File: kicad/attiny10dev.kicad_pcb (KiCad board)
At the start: 2 copper layers, 19 parts, among them J1 Conn_02x06_Odd_Even, J2 Conn_01x06, J3 Conn_01x03_Male, K1 m4-12h, K2 m4-12h, Q1 2N7002, Q2 BSS84, Q3 2N7002, Q4 FZT600, Q5 2N7002, U1 ATtiny10-TS, U2 ATtiny10-TS

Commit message: Work on next gen pcb
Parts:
- added C10: 100n, Capacitor_SMD:C_0805_2012Metric_Pad1.15x1.40mm_HandSolder, F.Cu at (239.3, 85.1)
- added C11: 500p, Capacitor_SMD:C_0805_2012Metric_Pad1.15x1.40mm_HandSolder, F.Cu at (259.4, 81.6)
- added C12: 470u, Capacitor_THT:CP_Radial_D8.0mm_P5.00mm, F.Cu at (254.3, 105.8)
- added C4: 1u, Capacitor_SMD:C_0805_2012Metric_Pad1.15x1.40mm_HandSolder, F.Cu at (233.8, 92.5)
- added C5: 100n, Capacitor_SMD:C_0805_2012Metric_Pad1.15x1.40mm_HandSolder, F.Cu at (243.7, 67.6)
- added C6: 100n, Capacitor_SMD:C_0805_2012Metric_Pad1.15x1.40mm_HandSolder, F.Cu at (250.8, 96.8)
- added C7: 100n, Capacitor_SMD:C_0805_2012Metric_Pad1.15x1.40mm_HandSolder, F.Cu at (246.6, 85.2)
- added C8: 100n, Capacitor_SMD:C_0805_2012Metric_Pad1.15x1.40mm_HandSolder, F.Cu at (237.6, 101.1)
- added C9: 470u, Capacitor_THT:CP_Radial_D8.0mm_P5.00mm, F.Cu at (263.6, 105.8)
- added D2: D, Diode_SMD:D_3220_8050Metric_Pad2.65x5.15mm_HandSolder, F.Cu at (259.5, 89.8)
- added F1: 500ma, Fuse:Fuse_1206_3216Metric_Pad1.42x1.75mm_HandSolder, F.Cu at (231.2, 95.9)
- added L1: 33u, Inductor_THT:L_Toroid_Vertical_L13.0mm_W6.5mm_P5.60mm, F.Cu at (272.8, 91.5)
- added R10: 10k, Capacitor_SMD:C_0603_1608Metric_Pad1.05x0.95mm_HandSolder, F.Cu at (254.2, 97.8)
- added R4: 10k, Capacitor_SMD:C_0603_1608Metric_Pad1.05x0.95mm_HandSolder, F.Cu at (217.7, 105.5)
- added R5: 22, Capacitor_SMD:C_0603_1608Metric_Pad1.05x0.95mm_HandSolder, F.Cu at (229.6, 90.7)
- added R6: 22, Capacitor_SMD:C_0603_1608Metric_Pad1.05x0.95mm_HandSolder, F.Cu at (229.6, 89.0)
- added R7: 470m, Resistor_THT:R_Axial_DIN0204_L3.6mm_D1.6mm_P2.54mm_Vertical, F.Cu at (258.3, 97.6)
- added R8: 180, Capacitor_SMD:C_0603_1608Metric_Pad1.05x0.95mm_HandSolder, F.Cu at (263.8, 98.6)
- added R9: 86k, Capacitor_SMD:C_0603_1608Metric_Pad1.05x0.95mm_HandSolder, F.Cu at (256.0, 97.8)
- added SW1: SW_Push, Button_Switch_THT:SW_PUSH_6mm, F.Cu at (220.2, 101.5)
- added U3: ATmega32U4-AU, Package_QFP:TQFP-44_10x10mm_P0.8mm, F.Cu at (243.0, 93.0)
- added U4: MC34063AD, Package_DIP:DIP-8_W10.16mm, F.Cu at (263.3, 84.7)
- added Y1: 16Mhz, Crystal:Crystal_SMD_HC49-SD, F.Cu at (242.9, 104.9)
- C2, C3: value 22u -> 22p; footprint Capacitor_THT:CP_Radial_D12.5mm_P5.00mm -> Capacitor_SMD:C_0805_2012Metric_Pad1.15x1.40mm_HandSolder; moved to F.Cu
- D1, J1, K1, K2, U2: moved to F.Cu
- J2: value Conn_01x06 -> Conn_02x03_Odd_Even; footprint Connector_PinHeader_2.54mm:PinHeader_1x06_P2.54mm_Vertical -> Connector_PinHeader_2.54mm:PinHeader_2x03_P2.54mm_Vertical; moved to F.Cu
- J3: value Conn_01x03_Male -> USB_B; footprint TerminalBlock_RND:TerminalBlock_RND_205-00277_1x03_P5.00mm_Vertical -> Connector_USB:USB_B_OST_USB-B1HSxx_Horizontal; moved to F.Cu
- Q4: value FZT600 -> 2N7002; footprint Package_TO_SOT_THT:TO-92 -> Package_TO_SOT_SMD:SOT-23; moved to F.Cu
- R1, R2, R3: footprint Resistor_SMD:R_0805_2012Metric_Pad1.15x1.40mm_HandSolder -> Capacitor_SMD:C_0603_1608Metric_Pad1.05x0.95mm_HandSolder
- moved K2 216.4 mm to (268.6, 69.3), turned to 0 degrees
- moved J2 194.5 mm to (231.1, 100.2)
- moved C3 193.4 mm to (241.1, 101.1)
- moved Q5 192.8 mm to (232.0, 80.2), turned to 90 degrees
- moved K1 191.9 mm to (256.2, 69.9), turned to 0 degrees
- moved R1 190.4 mm to (229.3, 76.4), turned to 270 degrees
- moved R3 188.3 mm to (232.2, 77.0), turned to 180 degrees
- moved Q1 185.6 mm to (223.8, 80.3), turned to 90 degrees
- moved Q3 185.5 mm to (228.0, 80.3), turned to 0 degrees
- moved Q2 183.8 mm to (226.2, 76.5), turned to 180 degrees
- moved C1 179.5 mm to (259.3, 100.1), turned to 0 degrees
- moved D1 175.2 mm to (231.6, 74.7), turned to 0 degrees
- moved C2 175.2 mm to (244.6, 101.1)
- moved Q4 171.3 mm to (236.1, 78.2), turned to 90 degrees
- moved J3 168.1 mm to (224.8, 92.2), turned to 180 degrees
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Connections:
- C2 pad 1: GND -> Net-(C2-Pad1)
- C2 pad 2: +5V -> GND
- C3 pad 1: GND -> Net-(C3-Pad1)
- C3 pad 2: +12V -> GND
- J2 pad 1: /tpidata -> /prog_miso
- J2 pad 2: /tpiclk -> +5V
- J2 pad 3: /prog -> /prog_sck
- J2 pad 4: /hard_reset -> /prog_mosi
- J2 pad 5: /reset_low -> /prog_rst
- J3 pad 1: +12V -> Net-(F1-Pad1)
- J3 pad 2: GND -> Net-(J3-Pad2)
- J3 pad 3: +5V -> Net-(J3-Pad3)
- K1 pad 1: /lower_relay -> +12V
- K1 pad 10: +12V -> /lower_relay
- K1 pad 5: /tpiclk -> /tpi_clk
- K1 pad 6: /tpidata -> /tpi_data
- Q4 pad 1: GND -> /prog
- Q4 pad 2: Net-(Q4-Pad2) -> GND
- R2 pad 1: Net-(Q4-Pad2) -> /prog
- R2 pad 2: /prog -> GND
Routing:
- net /io3: track 58.3 -> 0.00 mm
- net +12V: track 55.2 -> 0.00 mm
- net /pb3: track 45.2 -> 0.00 mm
- net +5V: track 100.4 -> 55.7 mm, vias 1 -> 0
- net Net-(K2-Pad5): track 44.1 -> 0.00 mm, vias 2 -> 0
- net /prog: track 40.7 -> 0.00 mm
- net /pb1: track 35.6 -> 0.00 mm
- net /io0: track 34.9 -> 0.00 mm
- net /pb0: track 33.3 -> 0.00 mm
- net /lower_relay: track 31.7 -> 0.00 mm
- net /tpiclk: track 31.0 -> 0.00 mm
- net /io1: track 26.2 -> 0.00 mm
- net /hard_reset: track 25.9 -> 0.00 mm
- net /tpidata: track 23.2 -> 0.00 mm
- net /reset_low: track 18.6 -> 0.00 mm
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- removed copper zone on B.Cu, net GND
- removed copper zone on F.Cu, net GND
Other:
- net class Default: via_dia 1.5 -> 0.8
- board text removed: "."
- board text removed: "ATtiny10 V4"
- board text removed: "Anton Lööf"
- board text removed: "gnd +5 io3 io2 io1 io0"
- board text removed: "gnd rst0 rst1 prog tclk tdat"

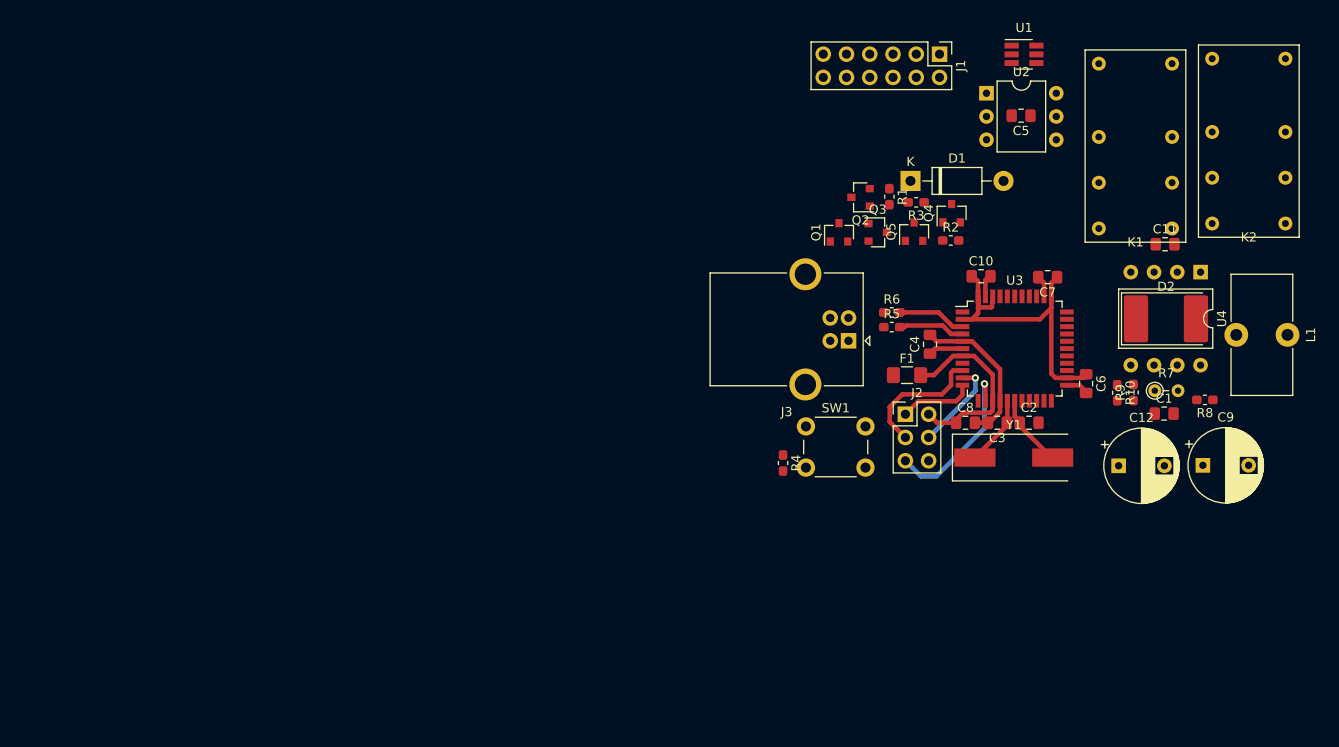
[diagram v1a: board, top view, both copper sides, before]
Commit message: V2 of pcb
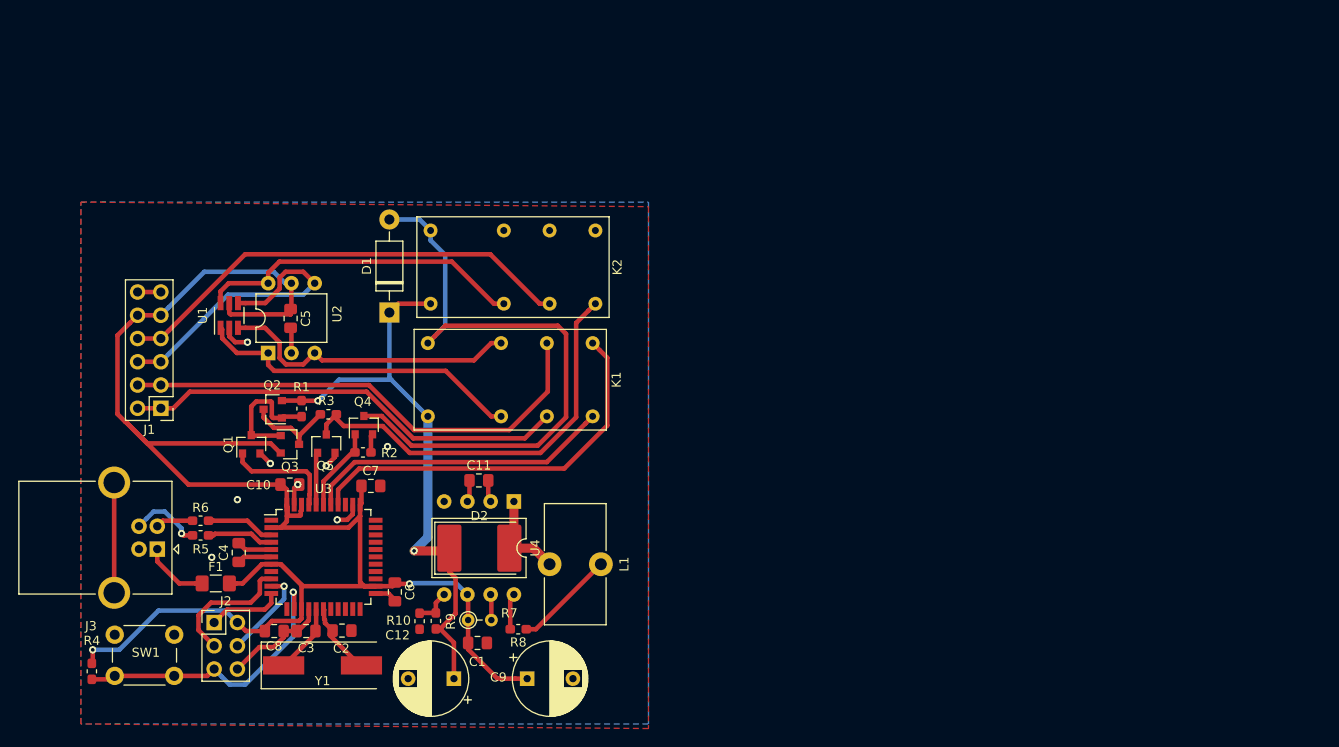
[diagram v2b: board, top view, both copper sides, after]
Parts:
- moved J1 93.4 mm to (149.7, 99.5), turned to 180 degrees
- moved U1 91.4 mm to (157.2, 89.4), turned to 90 degrees
- moved U2 83.4 mm to (161.5, 93.5), turned to 90 degrees
- moved C5 82.8 mm to (163.9, 89.7), turned to 270 degrees
- moved K2 82.7 mm to (187.2, 84.1), turned to 90 degrees
- moved R10 80.2 mm to (178.0, 122.8)
- moved R9 80.2 mm to (179.8, 122.7)
- moved C11 79.3 mm to (184.5, 107.4)
- moved C1 79.1 mm to (184.3, 125.2)
- moved L1 79.1 mm to (197.8, 116.5)
- moved R7 79.1 mm to (183.3, 122.7)
- moved U4 79.1 mm to (188.3, 109.7)
- moved D2 79.1 mm to (184.5, 114.8)
- moved R8 79.1 mm to (188.8, 123.7)
- moved C10 78.9 mm to (163.8, 107.8)
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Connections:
- K1 pad 3: /pb1 -> /pb0
- K1 pad 4: /io1 -> /io0
- K1 pad 5: /tpi_clk -> /tpi_data
- K1 pad 6: /tpi_data -> /tpi_clk
- K1 pad 7: /io0 -> /io1
- K1 pad 8: /pb0 -> /pb1
- U3 pad 37: /prog -> /tpi_clk
- U3 pad 38: /tpi_clk -> /tpi_data
- U3 pad 39: /tpi_data -> /prog
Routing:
- net +5V: track 55.7 -> 190.2 mm, vias 0 -> 2
- net /lower_relay: track 0.00 -> 68.8 mm
- net +12V: track 0.00 -> 66.5 mm, vias 0 -> 2
- net /io1: track 0.00 -> 54.0 mm
- net /io3: track 0.00 -> 51.0 mm
- net /io0: track 0.00 -> 48.6 mm
- net Net-(K2-Pad5): track 0.00 -> 45.8 mm
- net /tpi_clk: track 0.00 -> 43.6 mm
- net /pb3: track 0.00 -> 36.1 mm
- net /pb0: track 0.00 -> 36.0 mm
- net /io2: track 0.00 -> 33.9 mm
- net /tpi_data: track 0.00 -> 33.8 mm
- net /pb1: track 0.00 -> 33.0 mm
- net GND: track 24.4 -> 39.9 mm, vias 0 -> 8
- net /prog_rst: track 18.3 -> 32.1 mm
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- added copper zone on B.Cu, net GND
- added copper zone on F.Cu, net GND
